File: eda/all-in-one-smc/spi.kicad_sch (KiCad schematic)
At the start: 13 parts, among them U23 74HCT14, U24 74HCT86, U26 74HCT595, U27 74HCT165, U31 74HCT138

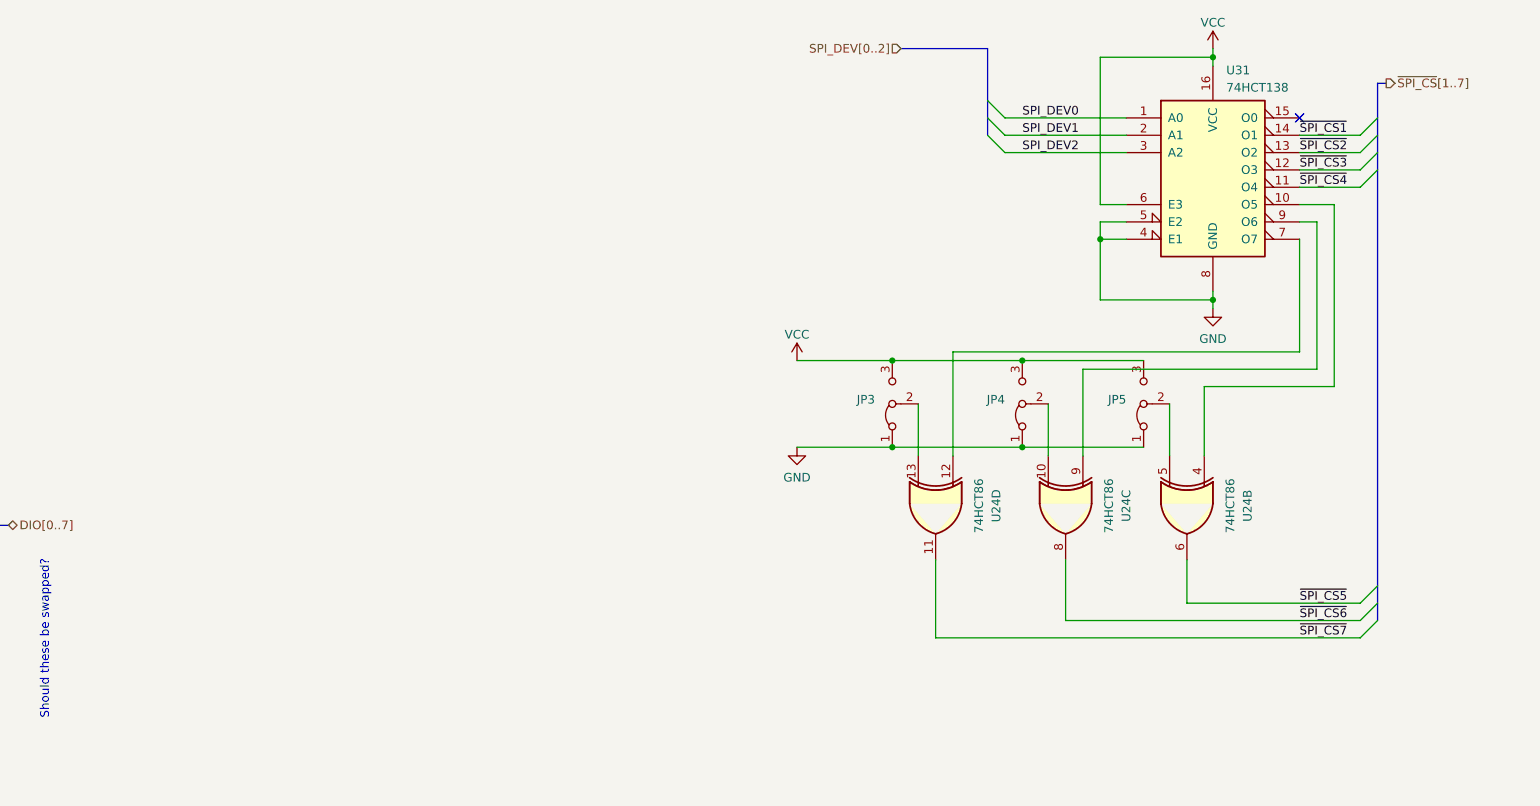
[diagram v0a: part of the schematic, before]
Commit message: wip
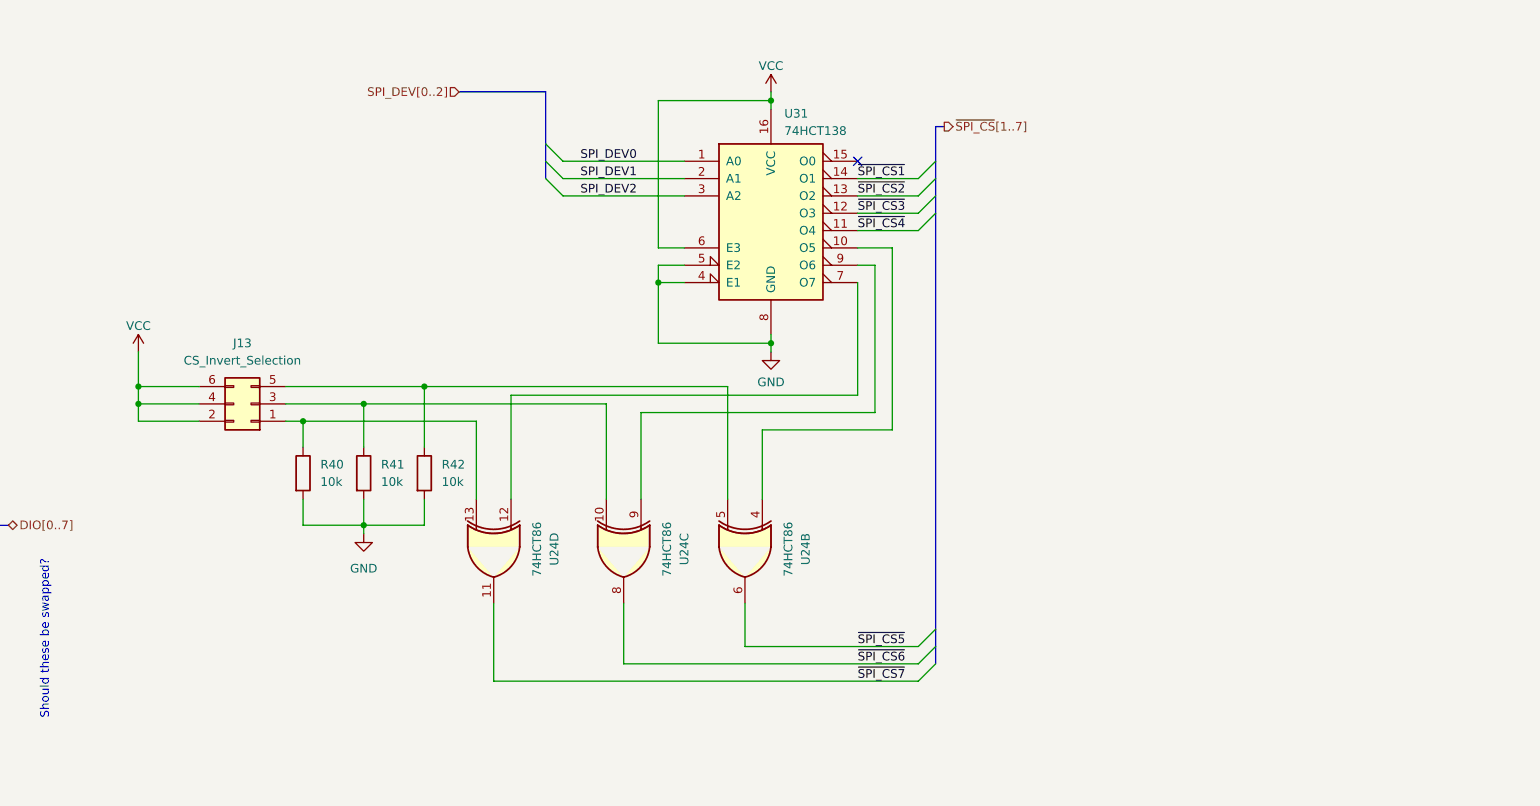
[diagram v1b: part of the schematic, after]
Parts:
- removed JP3, JP4, JP5: ~, Connector_PinHeader_2.54mm:PinHeader_1x03_P2.54mm_Vertical, symbol Jumper:Jumper_3_Bridged12
- added J13: CS_Invert_Selection, Connector_PinHeader_2.54mm:PinHeader_2x03_P2.54mm_Horizontal, symbol Connector_Generic:Conn_02x03_Odd_Even
- added R40, R41, R42: 10k, Resistor_SMD:R_0805_2012Metric, symbol Device:R
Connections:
- net GND: now also R40.2, R41.2, R42.2
- net VCC: now also J13.2 (Pin_2), J13.4 (Pin_4), J13.6 (Pin_6)
- net at U24.5: now also J13.5 (Pin_5), R42.1
- net at U24.13: now also J13.1 (Pin_1), R40.1
- net at U24.10: now also J13.3 (Pin_3), R41.1
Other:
- moved on the sheet: U24B, U24C, U24D, U31
